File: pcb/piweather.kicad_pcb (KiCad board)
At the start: 4 copper layers, 35 x 35 mm, 70 parts, among them J1 USB_B_Micro, J3 CONN127P-02X13-M55-7012642R, J5 CONN_01X03, U1 STM32F405RGTx, U2 AP3418, U3 SN65HVD232D, U4 AS5047P, Y1 Crystal_GND24

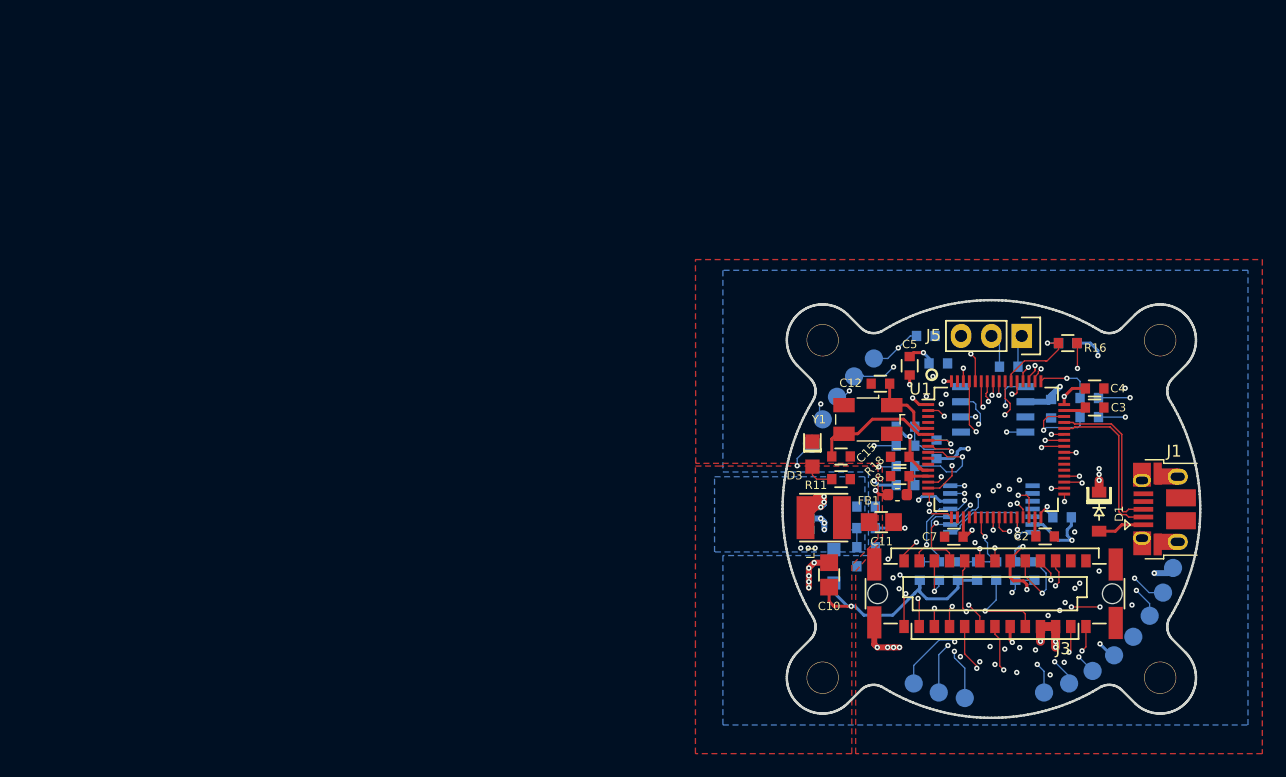
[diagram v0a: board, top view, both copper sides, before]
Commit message: wip
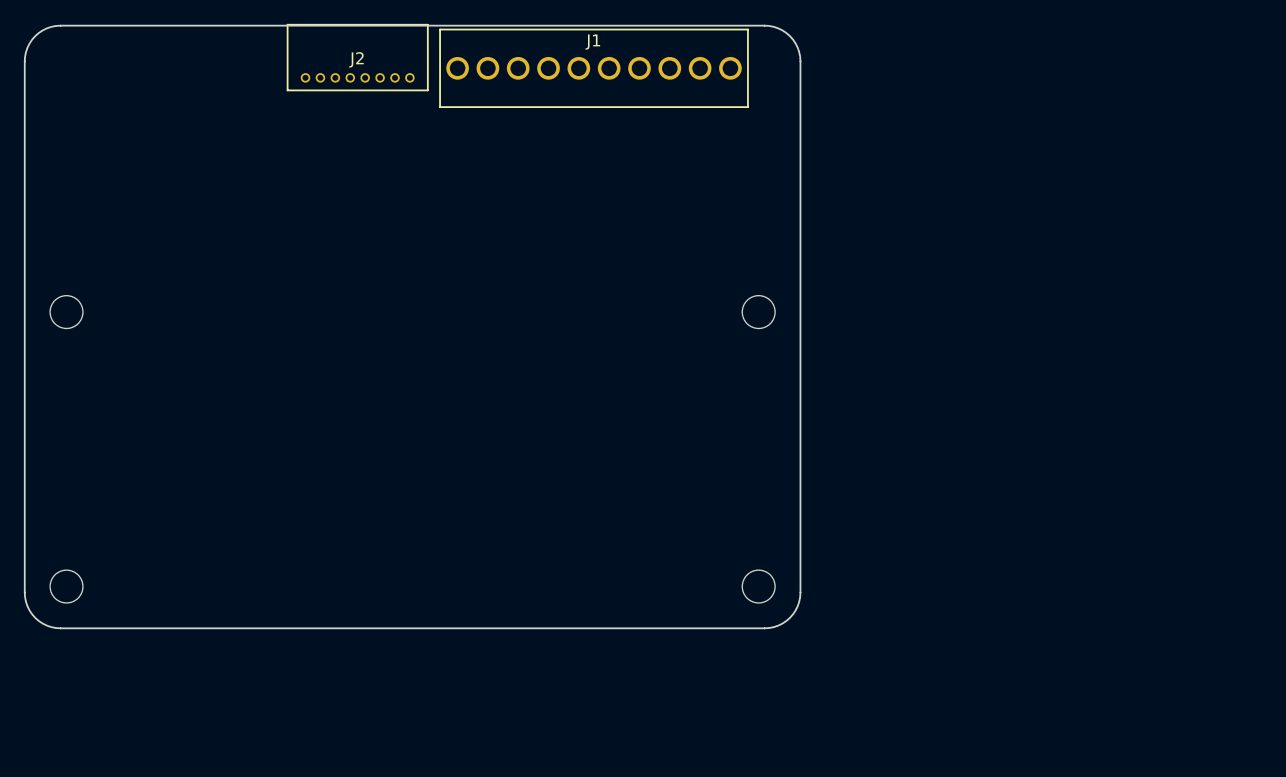
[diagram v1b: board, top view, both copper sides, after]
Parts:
- removed C1: CC0603JRNPO8BN102, Main:CAPC0603
- removed C10, C11: CC0805MKX5R5BB226, Main:CAPC0805
- removed C12, C15: CC0603JRNPO9BN100, Main:CAPC0603
- removed C13, C14, C16, C21, C4, C5, C6, C7, C8: CC0603KRX7R7BB104, Main:CAPC0603
- removed C17, C18: CC0603KRX7R9BB222, Main:CAPC0603
- removed C19, C20: CC0603JRNPO9BN470, Main:CAPC0603
- removed C2, C3: CC0603KRX5R5BB225, Main:CAPC0603
- removed C9: CC0603KRX5R5BB475, Main:CAPC0603
- removed D1: MBR0520LT1G, Main:SOD3717X135
- removed D2: SMF, Diode_SMD:D_SOD-123F
- removed D3: LTW-170TK, Main:DIOC200X120X110
- removed FB1: Ferrite_Bead, Capacitor_SMD:C_0603_1608Metric
- removed J3: CONN127P-02X13-M55-7012642R, Main:CONN127P-02X13-M55-7012642R
- removed J5: CONN_01X03, Main:SOCKET254P-01X03
- removed L1: INDUCTOR_SRN4026-2R2Y, Main:INDP400400X250
- removed R1: RC0603FR-0710RL, Main:RESC0603
- removed R11, R12, R13, R5, R6: RC0603FR-0722R1L, Main:RESC0603
- removed R14, R8: RC0603FR-07100KL, Main:RESC0603
- removed R15, R16, R17: RC0603FR-07499RL, Main:RESC0603
- removed R18: RC0603FR-070RL, Main:RESC0603
- removed R2: RC0603FR-0727K4L, Main:RESC0603
- removed R3: RC0603FR-076K04L, Main:RESC0603
- removed R4: RC0603FR-07121RL, Main:RESC0603
- removed R9: RC0603FR-0710KL, Main:RESC0603
- removed TP11, TP12, TP13, TP14, TP15, TP16, TP17, TP18, TP19, TP2, TP3, TP4, TP5, TP6, TP8, TP9: TestPoint, Main:TestPoint000
- removed U1: STM32F405RGTx, Package_QFP:LQFP-64_10x10mm_P0.5mm
- removed U2: AP3418, Main:SOT095P300X150X145-5
- removed U3: SN65HVD232D, Main:SOIC127P490X390X175-8
- removed U4: AS5047P, Package_SO:SSOP-14_5.3x6.2mm_P0.65mm
- removed Y1: Crystal_GND24, Crystal:Crystal_SMD_Abracon_ABM3B-4Pin_5.0x3.2mm
- added J2: Conn_01x08_Male, Main:PICOBLADE_FEMALE_8, F.Cu at (95.4, 68.9)
- H1, H2, H3, H4: footprint Main:MECH_NPTH_M3 -> Main:RPi_Hat_Mounting_Hole
- J1: value USB_B_Micro -> Screw_Terminal_01x10; footprint Connector_USB:USB_Micro-B_Amphenol_10103594-0001LF_Horizontal -> Main:Terminal_block_OSTVN10A150
- moved H2 92.0 mm to (71.0, 111.5)
- moved H1 63.4 mm to (71.0, 88.5)
- moved J1 60.4 mm to (115.2, 68.1), turned to 180 degrees
- moved H4 33.7 mm to (129.0, 88.5)
- moved H3 9.33 mm to (129.0, 111.5)
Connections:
- J1 pad 1: /USB_VBUS -> (no net)
- J1 pad 2: /USB_D_N -> (no net)
- J1 pad 3: /USB_D_P -> (no net)
- J1 pad 5: GND -> (no net)
- J1 pad 6: GND -> (no net)
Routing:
- net GNDA: track 75.3 -> 0.00 mm, vias 6 -> 0
- net GND: track 54.0 -> 0.00 mm, vias 16 -> 0
- net /nFAULT_C: track 46.2 -> 0.00 mm, vias 6 -> 0
- net /GPIO7: track 37.6 -> 0.00 mm, vias 3 -> 0
- net +5V: track 36.4 -> 0.00 mm, vias 11 -> 0
- net /M0_CH: track 33.9 -> 0.00 mm, vias 3 -> 0
- net /I2C1_SCL: track 33.7 -> 0.00 mm, vias 4 -> 0
- net /I2C1_SDA: track 33.4 -> 0.00 mm, vias 5 -> 0
- net /nRST: track 33.1 -> 0.00 mm, vias 3 -> 0
- net /GPIO8: track 32.3 -> 0.00 mm, vias 3 -> 0
- net /M0_AH: track 31.0 -> 0.00 mm, vias 3 -> 0
- net /M0_SO1_C: track 30.6 -> 0.00 mm, vias 3 -> 0
- net /M0_CL: track 29.4 -> 0.00 mm, vias 3 -> 0
- net /M0_BL: track 28.1 -> 0.00 mm, vias 3 -> 0
- net /M0_BH: track 27.0 -> 0.00 mm, vias 3 -> 0
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- removed copper zone on B.Cu, net +3V3
- removed copper zone on F.Cu, net +3V3
- removed copper zone on B.Cu, net +5V
- removed copper zone on In2.Cu, net +5V
- removed copper zone on F.Cu, net GND
- removed copper zone on In1.Cu, net GND
- removed copper zone on In2.Cu, net GND
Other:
- board size 35 x 35 mm -> 65 x 50.5 mm
- board text removed: "3V3"
- board text removed: "5V"
- board text removed: "BOOT0"
- board text removed: "Board center X148.5 Y105"
- board text removed: "DIR"
- board text removed: "GND"
- board text removed: "GPIO5"
- board text removed: "GPIO7"
- board text removed: "GPIO8"
- board text removed: "I2C1_SCL"
- board text removed: "I2C1_SDA"
- board text removed: "RX"
- board text removed: "STEP"
- board text removed: "SWCLK"
- board text removed: "SWDIO"
- board text removed: "TX"
- board text removed: "~RST"
